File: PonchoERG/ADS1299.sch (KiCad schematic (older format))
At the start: 13 parts, among them J2 I/O's Multi Propósito, U10 ADS1299

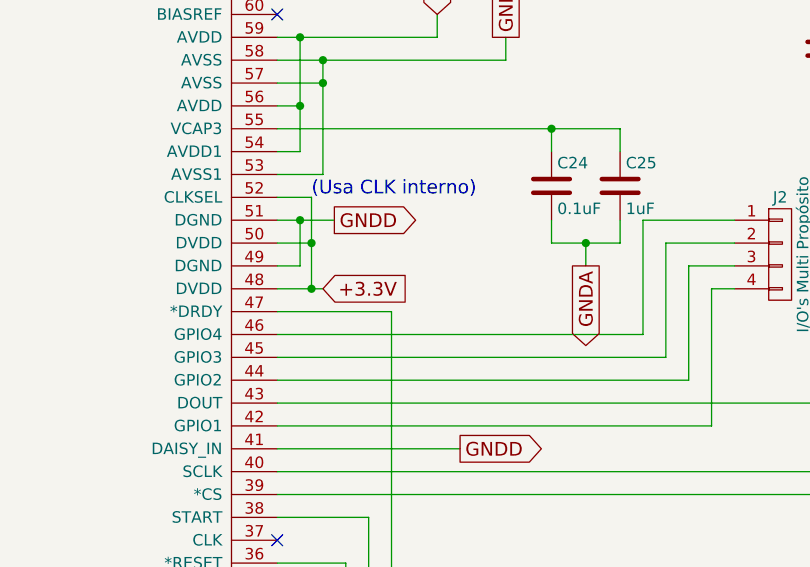
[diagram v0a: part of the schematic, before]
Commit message: Subida n.0
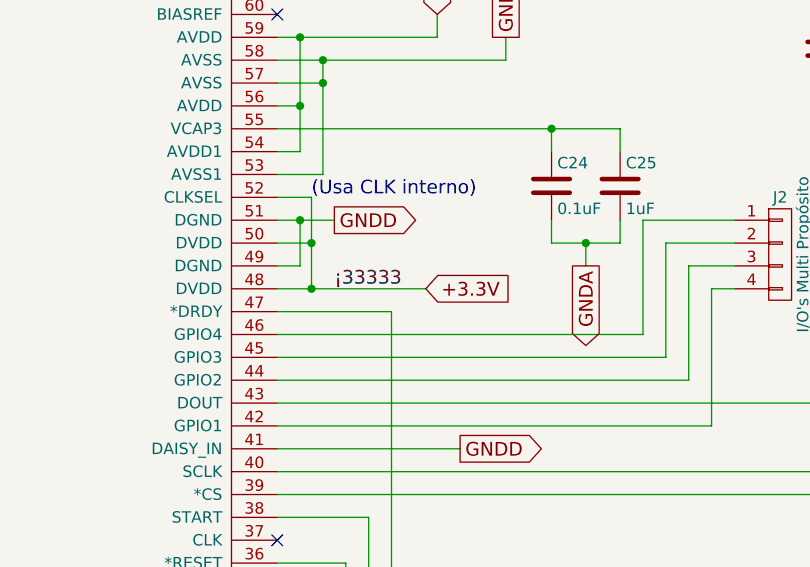
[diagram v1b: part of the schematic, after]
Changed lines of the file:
@@
 	3900 5100 4600 5100
 Wire Wire Line
-	6400 3800 6600 3800
+	6400 3800 7050 3800
 Wire Wire Line
 	6400 3600 6550 3600
@@
 Text GLabel 3700 3700 1    60   Input ~ 0
 +3.3V
-Text GLabel 6600 3800 2    60   Input ~ 0
+Text GLabel 7050 3800 2    60   Input ~ 0
 +3.3V
 Text GLabel 7200 5100 2    60   Input ~ 0
@@
 Text GLabel 9900 2400 1    60   Input ~ 0
 +5V
+Text Label 6650 3800 0    60   ~ 0
+¡33333
 $EndSCHEMATC
